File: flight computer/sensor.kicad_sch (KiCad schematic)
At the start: 92 parts, among them J1 Micro_SD_Card_Det1, J12 Conn_01x04, J13 1x3 servo, J14 1x3 servo, J15 arming terminal, J16 arming terminal, J17 H9161TR-ND, J19 Screw_Terminal_01x02, J20 Screw_Terminal_01x02, J3 H9161TR-ND, J4 H9161TR-ND, J5 Screw_Term, J6 1x3 servo, J9 1x3 servo, Q7 BSS138, Q8 IRLML6402, Q9 IRLML6402, U10 LSM6DS3, U11 BGM220SC12WGA2R, U16 SX1262IMLTRT, U17 PE4259, U5 LPS22HB, U6 GPS, U8 NAND, Y2 32MHz

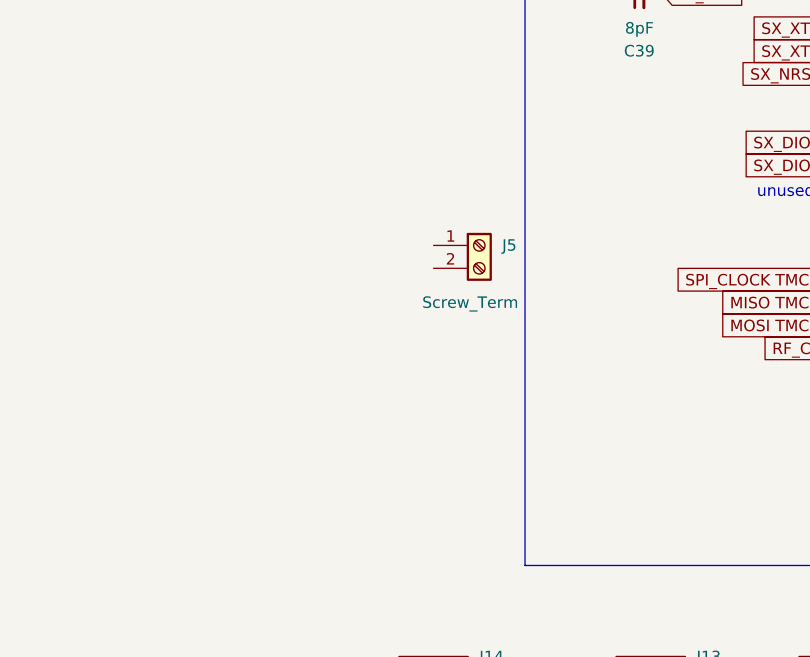
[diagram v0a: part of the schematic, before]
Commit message: push
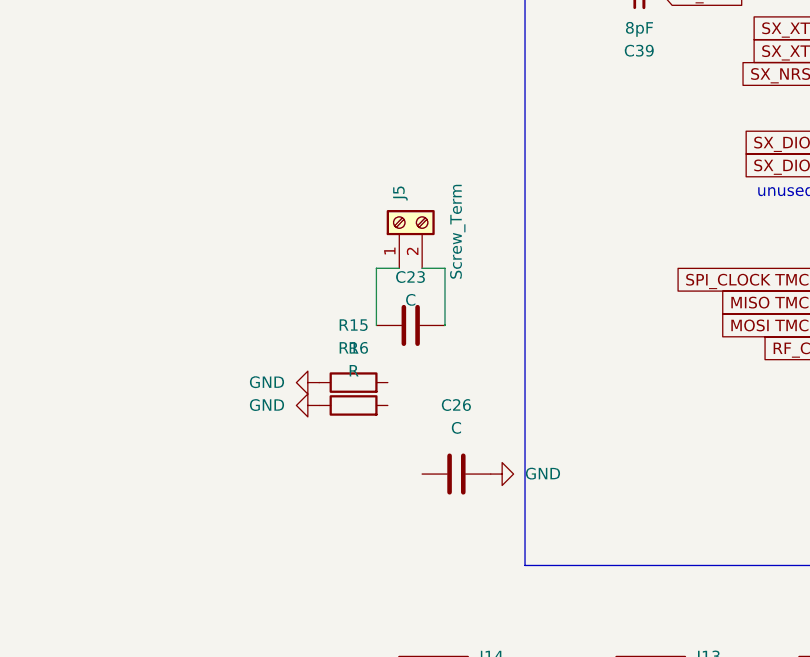
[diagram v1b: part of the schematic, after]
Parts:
- added C23, C26: C, symbol Device:C
- added R15, R16: R, symbol Device:R
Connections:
- net GND: now also C26.2, R15.1, R16.1
- net at J5.1 (Pin_1): now also C23.1
- net at J5.2 (Pin_2): now also C23.2
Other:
- moved on the sheet: J5
